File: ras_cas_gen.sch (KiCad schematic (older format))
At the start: 13 parts, among them U3 74HCT02, U4 NE555, U5 74HCT573, U6 74HCT245, U7 GAL20V8

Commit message: Ready for V1
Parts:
- U5, U6: footprint Package_SO:SOIC-20W_7.5x12.8mm_P1.27mm -> Package_SO:SO-20_5.3x12.6mm_P1.27mm
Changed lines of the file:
@@
 F 0 "U5" H 6255 6915 50  0000 C CNN
 F 1 "74HCT573" H 6315 5585 50  0000 C CNN
-F 2 "Package_SO:SOIC-20W_7.5x12.8mm_P1.27mm" H 6055 6265 50  0001 C CNN
+F 2 "Package_SO:SO-20_5.3x12.6mm_P1.27mm" H 6055 6265 50  0001 C CNN
 F 3 "74xx/74hc573.pdf" H 6055 6265 50  0001 C CNN
 F 4 "595-SN74HCT573NSR" H 6055 6265 50  0001 C CNN "MouserPN"
@@
 F 0 "U6" H 11790 8140 50  0000 C CNN
 F 1 "74HCT245" H 11800 6830 50  0000 C CNN
-F 2 "Package_SO:SOIC-20W_7.5x12.8mm_P1.27mm" H 11575 7495 50  0001 C CNN
+F 2 "Package_SO:SO-20_5.3x12.6mm_P1.27mm" H 11575 7495 50  0001 C CNN
 F 3 "http://www.ti.com/lit/gpn/sn74LS245" H 11575 7495 50  0001 C CNN
 F 4 "595-SN74HCT245ANSR" H 11575 7495 50  0001 C CNN "MouserPN"
@@
 Text GLabel 7850 9925 2    50   Output ~ 0
 ~SRAM_CE
-Wire Bus Line
-	7590 2250 7590 3360
-Wire Bus Line
-	7590 3660 7590 4535
-Wire Bus Line
-	12440 7095 12440 7795
-Wire Bus Line
-	4990 5865 4990 6565
-Wire Bus Line
-	7925 5865 7925 6565
-Wire Bus Line
-	10460 6895 10460 7595
-Wire Bus Line
-	5090 2250 5090 3460
 $Comp
 L Device:C C?
@@
 	1    0    0    -1
 $EndComp
+Wire Bus Line
+	7590 2250 7590 3360
+Wire Bus Line
+	7590 3660 7590 4535
+Wire Bus Line
+	12440 7095 12440 7795
+Wire Bus Line
+	4990 5865 4990 6565
+Wire Bus Line
+	7925 5865 7925 6565
+Wire Bus Line
+	10460 6895 10460 7595
+Wire Bus Line
+	5090 2250 5090 3460
 $EndSCHEMATC

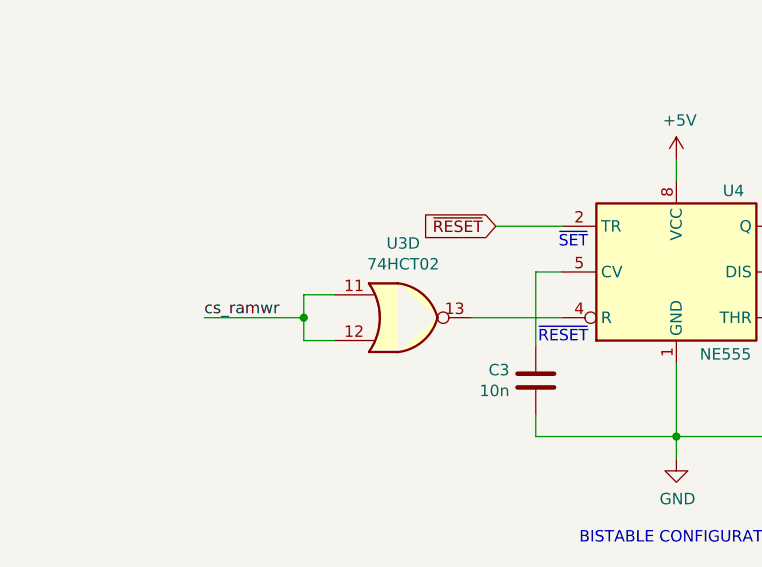
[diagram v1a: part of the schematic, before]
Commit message: More rerouting
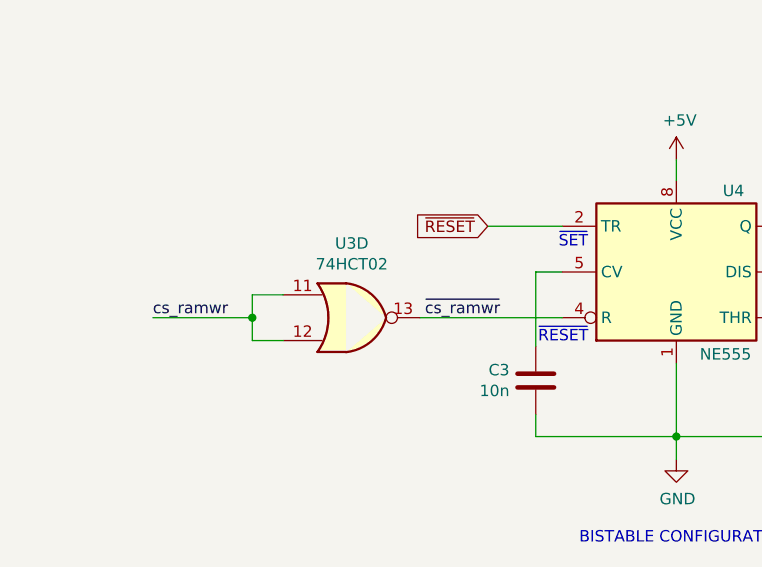
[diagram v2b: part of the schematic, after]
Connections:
- net ~cs_ramwr: now reaches U3.13, U4.4 (R)
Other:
- moved on the sheet: U3D
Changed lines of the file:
@@
 	2905 7350 2905 7675
 Wire Wire Line
-	3020 7550 2625 7550
-Wire Wire Line
-	3020 7150 2730 7150
+	3020 7150 2695 7150
 NoConn ~ 4020 7350
 Text Notes 3005 7250 0    50   ~ 0
@@
 Wire Wire Line
 	4990 7150 4020 7150
-Text GLabel 2730 7150 0    50   Input ~ 0
+Text GLabel 2695 7150 0    50   Input ~ 0
 ~RESET
-Text Label 1455 7550 0    50   ~ 0
+Text Label 1230 7550 0    50   ~ 0
 cs_ramwr
 Text Notes 3095 8545 0    50   ~ 0
@@
 L 74xx:74HCT02 U?
 U 4 1 641A3A3A
-P 2325 7550
+P 2100 7550
 AR Path="/62E48B71/641A3A3A" Ref="U?"  Part="4"
 AR Path="/63A22C28/641A3A3A" Ref="U3"  Part="4"
-F 0 "U3" H 2325 7875 50  0000 C CNN
-F 1 "74HCT02" H 2325 7784 50  0000 C CNN
-F 2 "Package_SO:SOIC-14_3.9x8.7mm_P1.27mm" H 2325 7550 50  0001 C CNN
-F 3 "http://www.ti.com/lit/gpn/sn74hct02" H 2325 7550 50  0001 C CNN
-	4    2325 7550
-	1    0    0    -1
-$EndComp
-Wire Wire Line
-	2025 7450 1890 7450
-Wire Wire Line
-	1890 7450 1890 7550
-Wire Wire Line
-	1890 7650 2025 7650
-Wire Wire Line
-	1890 7550 1455 7550
-Connection ~ 1890 7550
-Wire Wire Line
-	1890 7550 1890 7650
+F 0 "U3" H 2100 7875 50  0000 C CNN
+F 1 "74HCT02" H 2100 7784 50  0000 C CNN
+F 2 "Package_SO:SOIC-14_3.9x8.7mm_P1.27mm" H 2100 7550 50  0001 C CNN
+F 3 "http://www.ti.com/lit/gpn/sn74hct02" H 2100 7550 50  0001 C CNN
+	4    2100 7550
+	1    0    0    -1
+$EndComp
+Wire Wire Line
+	1800 7450 1665 7450
+Wire Wire Line
+	1665 7450 1665 7550
+Wire Wire Line
+	1665 7650 1800 7650
+Wire Wire Line
+	1665 7550 1230 7550
+Connection ~ 1665 7550
+Wire Wire Line
+	1665 7550 1665 7650
 Text Notes 8095 3160 0    50   ~ 0
 $FD16 WRITE (NOTE: ACTIVE *HIGH*!)
@@
 	1    0    0    -1
 $EndComp
+Text Label 2420 7550 0    50   ~ 0
+~cs_ramwr
+Wire Wire Line
+	2400 7550 3020 7550
 Wire Bus Line
 	7590 2250 7590 3360

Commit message: Add part numbers
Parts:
- C2, C4, C5, C6, C7: LCSC (none) -> C49678
- C3: LCSC (none) -> C1710
- RN1, RN2: LCSC (none) -> C20197
- U3: LCSC (none) -> C471050; MouserPN (none) -> 771-74HCT02D-T
- U4: LCSC (none) -> C5125085
- U5: LCSC (none) -> C2864941
- U6: LCSC (none) -> C133641
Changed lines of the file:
@@
 F 2 "Capacitor_SMD:C_0805_2012Metric_Pad1.18x1.45mm_HandSolder" H 4453 3060 50  0001 C CNN
 F 3 "~" H 4415 3210 50  0001 C CNN
+F 4 "C49678" H 4415 3210 50  0001 C CNN "LCSC"
 	1    4415 3210
 	1    0    0    -1
@@
 F 2 "Capacitor_SMD:C_0805_2012Metric_Pad1.18x1.45mm_HandSolder" H 4628 5635 50  0001 C CNN
 F 3 "~" H 4590 5785 50  0001 C CNN
+F 4 "C49678" H 4590 5785 50  0001 C CNN "LCSC"
 	1    4590 5785
 	1    0    0    -1
@@
 F 3 "74xx/74hc573.pdf" H 6055 6265 50  0001 C CNN
 F 4 "595-SN74HCT573NSR" H 6055 6265 50  0001 C CNN "MouserPN"
+F 5 "C2864941" H 6055 6265 50  0001 C CNN "LCSC"
 	1    6055 6265
 	1    0    0    -1
@@
 F 2 "Package_SO:SOIC-8_3.9x4.9mm_P1.27mm" H 4370 6950 50  0001 C CNN
 F 3 "http://www.ti.com/lit/ds/symlink/ne555.pdf" H 4370 6950 50  0001 C CNN
+F 4 "C5125085" H 3520 7350 50  0001 C CNN "LCSC"
 	1    3520 7350
 	1    0    0    -1
@@
 F 2 "Capacitor_SMD:C_0805_2012Metric_Pad1.18x1.45mm_HandSolder" H 2943 7675 50  0001 C CNN
 F 3 "~" H 2905 7825 50  0001 C CNN
+F 4 "C1710" H 2905 7825 50  0001 C CNN "LCSC"
 	1    2905 7825
 	1    0    0    -1
@@
 F 2 "Resistor_SMD:R_Array_Convex_4x0603" V 7035 5425 50  0001 C CNN
 F 3 "~" H 6760 5425 50  0001 C CNN
+F 4 "C20197" H 6760 5425 50  0001 C CNN "LCSC"
 	1    6760 5425
 	-1   0    0    -1
@@
 F 2 "Resistor_SMD:R_Array_Convex_4x0603" V 7650 5425 50  0001 C CNN
 F 3 "~" H 7375 5425 50  0001 C CNN
+F 4 "C20197" H 7375 5425 50  0001 C CNN "LCSC"
 	1    7375 5425
 	-1   0    0    -1
@@
 F 3 "http://www.ti.com/lit/gpn/sn74LS245" H 11575 7495 50  0001 C CNN
 F 4 "595-SN74HCT245ANSR" H 11575 7495 50  0001 C CNN "MouserPN"
+F 5 "C133641" H 11575 7495 50  0001 C CNN "LCSC"
 	1    11575 7495
 	1    0    0    -1
@@
 F 2 "Capacitor_SMD:C_0805_2012Metric_Pad1.18x1.45mm_HandSolder" H 4688 7695 50  0001 C CNN
 F 3 "~" H 4650 7845 50  0001 C CNN
+F 4 "C49678" H 4650 7845 50  0001 C CNN "LCSC"
 	1    4650 7845
 	1    0    0    -1
@@
 F 2 "Package_SO:SOIC-14_3.9x8.7mm_P1.27mm" H 7315 9925 50  0001 C CNN
 F 3 "http://www.ti.com/lit/gpn/sn74hct02" H 7315 9925 50  0001 C CNN
+F 4 "C471050" H 7315 9925 50  0001 C CNN "LCSC"
+F 5 "771-74HCT02D-T" H 7315 9925 50  0001 C CNN "MouserPN"
 	1    7315 9925
 	1    0    0    -1
@@
 F 2 "Package_SO:SOIC-14_3.9x8.7mm_P1.27mm" H 6460 9925 50  0001 C CNN
 F 3 "http://www.ti.com/lit/gpn/sn74hct02" H 6460 9925 50  0001 C CNN
+F 4 "C471050" H 6460 9925 50  0001 C CNN "LCSC"
+F 5 "771-74HCT02D-T" H 6460 9925 50  0001 C CNN "MouserPN"
 	2    6460 9925
 	1    0    0    -1
@@
 F 2 "Package_SO:SOIC-14_3.9x8.7mm_P1.27mm" H 5400 9825 50  0001 C CNN
 F 3 "http://www.ti.com/lit/gpn/sn74hct02" H 5400 9825 50  0001 C CNN
+F 4 "C471050" H 5400 9825 50  0001 C CNN "LCSC"
+F 5 "771-74HCT02D-T" H 5400 9825 50  0001 C CNN "MouserPN"
 	3    5400 9825
 	1    0    0    -1
@@
 F 2 "Package_SO:SOIC-14_3.9x8.7mm_P1.27mm" H 845 10205 50  0001 C CNN
 F 3 "http://www.ti.com/lit/gpn/sn74hct02" H 845 10205 50  0001 C CNN
+F 4 "C471050" H 845 10205 50  0001 C CNN "LCSC"
+F 5 "771-74HCT02D-T" H 845 10205 50  0001 C CNN "MouserPN"
 	5    845  10205
 	1    0    0    -1
@@
 F 2 "Capacitor_SMD:C_0805_2012Metric_Pad1.18x1.45mm_HandSolder" H 1718 10050 50  0001 C CNN
 F 3 "~" H 1680 10200 50  0001 C CNN
+F 4 "C49678" H 1680 10200 50  0001 C CNN "LCSC"
 	1    1680 10200
 	1    0    0    -1
@@
 F 2 "Package_SO:SOIC-14_3.9x8.7mm_P1.27mm" H 2100 7550 50  0001 C CNN
 F 3 "http://www.ti.com/lit/gpn/sn74hct02" H 2100 7550 50  0001 C CNN
+F 4 "C471050" H 2100 7550 50  0001 C CNN "LCSC"
+F 5 "771-74HCT02D-T" H 2100 7550 50  0001 C CNN "MouserPN"
 	4    2100 7550
 	1    0    0    -1
@@
 F 2 "Capacitor_SMD:C_0805_2012Metric_Pad1.18x1.45mm_HandSolder" H 13068 6825 50  0001 C CNN
 F 3 "~" H 13030 6975 50  0001 C CNN
+F 4 "C49678" H 13030 6975 50  0001 C CNN "LCSC"
 	1    13030 6975
 	1    0    0    -1
